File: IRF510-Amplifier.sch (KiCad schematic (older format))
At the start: 37 parts, among them J1 Jack-DC, J2 BNC, J3 BNC, Q1 2N3904-SMD, Q2 2SC5706, Q4 IRF510, T1 T37-6 15T:7T, U6 MCP1703A-2502_SOT223

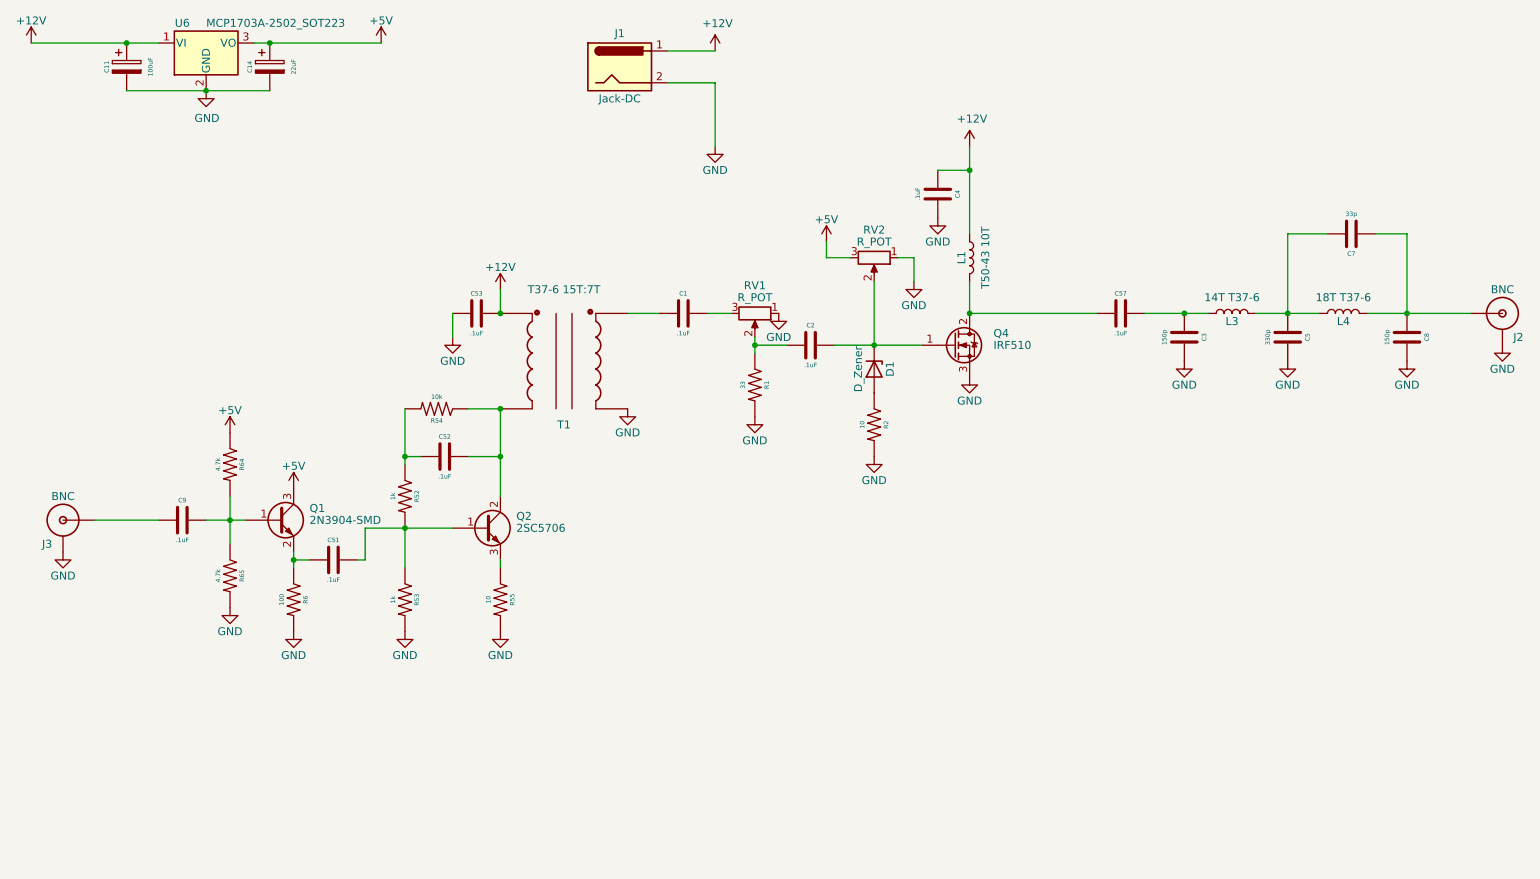
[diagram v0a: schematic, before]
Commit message: reorg
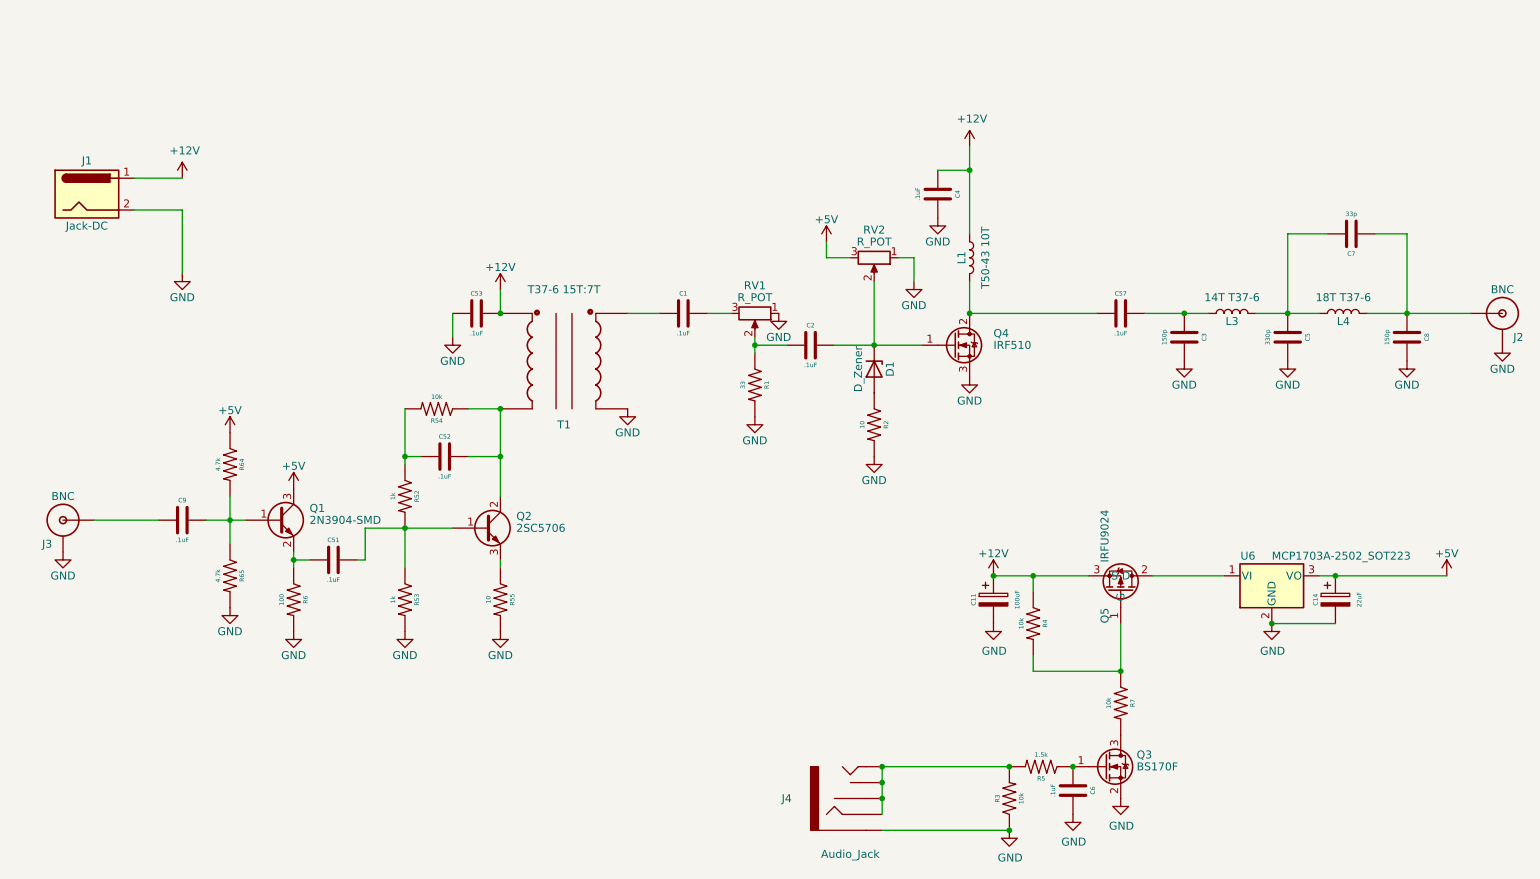
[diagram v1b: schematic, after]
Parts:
- added C6: .1uF, Xenir:Capacitor 0805, symbol Xenir:Capacitor
- added J4: Audio_Jack, Xenir:Audio_Jack, symbol Xenir:Audio_Jack
- added Q3: BS170F, Package_TO_SOT_SMD:SOT-23, symbol Transistor_FET:BS170F
- added Q5: IRFU9024, Package_TO_SOT_THT:TO-251-3_Vertical, symbol Xenir:IRFU9024
- added R3, R4, R7: 10k, Xenir:Resistor 0805, symbol Xenir:Resistor
- added R5: 1.5k, Xenir:Resistor 0805, symbol Xenir:Resistor
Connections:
- net +12V: now also Q5.3 (S), R4.1; no longer U6.1 (VI)
- net GND: now also C6.2, J4.SLEEVE, Q3.2 (S), R3.1
- new net: Q5.2 (D), U6.1 (VI)
- new net: Q5.1 (G), R4.2, R7.1
- new net: Q3.3 (D), R7.2
- new net: C6.1, Q3.1 (G), R5.1
- new net: J4.RING, J4.RSH, J4.TIP, J4.TSH, R3.2, R5.2
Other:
- moved on the sheet: C11, C14, J1, U6
